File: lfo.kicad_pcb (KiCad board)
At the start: 2 copper layers, 103.7 x 33.7 mm, 36 parts, among them J1 PJ398SM-12 (Tri), J2 PJ398SM-12 (square), J3 PJ398SM-12 (weird), J4 Conn_02x05_Odd_Even, Q1 BC547, SW1 SW_SPDT, U1 TL084

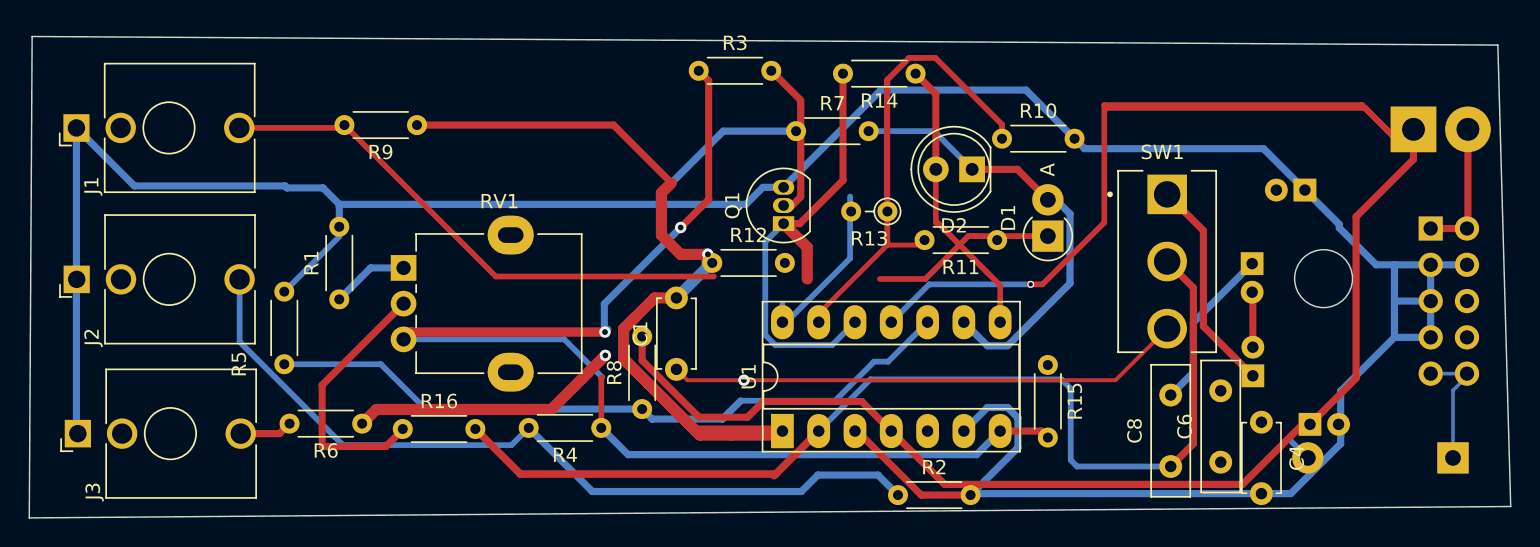
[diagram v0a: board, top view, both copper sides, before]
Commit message: successcive editing
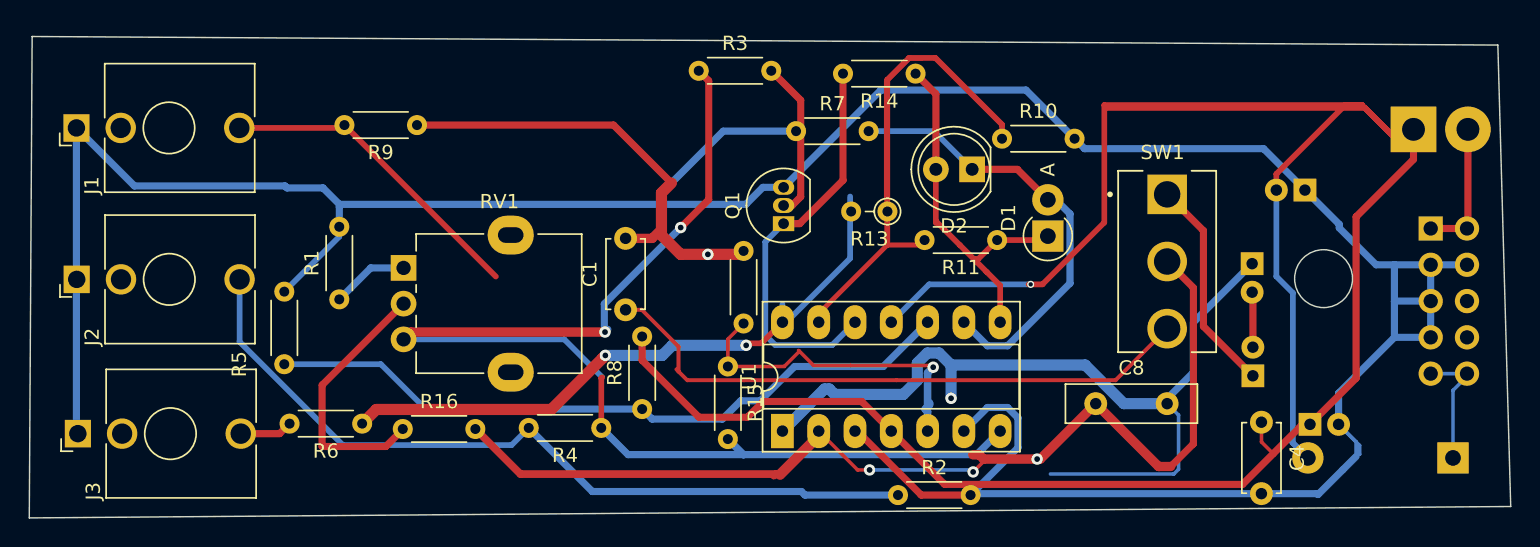
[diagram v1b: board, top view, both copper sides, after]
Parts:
- removed C6: 100nFC, Capacitor_THT:C_Disc_D9.0mm_W2.5mm_P5.00mm
- moved R15 22.4 mm to (105.8, 34.2)
- moved C8 6.85 mm to (131.6, 36.8), turned to 0 degrees
- moved C1 5.48 mm to (98.6, 30.2)
- moved R12 2.35 mm to (106.9, 26.1), turned to -90 degrees
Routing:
- net Vee: track 70.1 -> 98.9 mm
- net Net-(U1B-+): track 0.00 -> 24.3 mm, vias 0 -> 1
- net Net-(C1-Pad2): track 87.4 -> 103.0 mm, vias 1 -> 2
- net Net-(J1-PadT): track 37.7 -> 22.4 mm
- net Net-(R13-Pad2): track 31.2 -> 44.6 mm, vias 1 -> 2
- net Net-(D1-K): track 33.5 -> 25.8 mm
- net Net-(SW1-B): track 96.6 -> 103.7 mm, vias 0 -> 3
- net GND: track 215.5 -> 222.1 mm
- net Net-(SW1-C): track 36.2 -> 42.7 mm, vias 1 -> 0
- net Net-(Q1-C): track 33.0 -> 28.5 mm
- net Vcc: track 78.3 -> 80.9 mm
- net Net-(R15-Pad2): track 111.5 -> 109.5 mm
- net Net-(J2-PadT): track 56.9 -> 55.9 mm

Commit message: fix drc errors
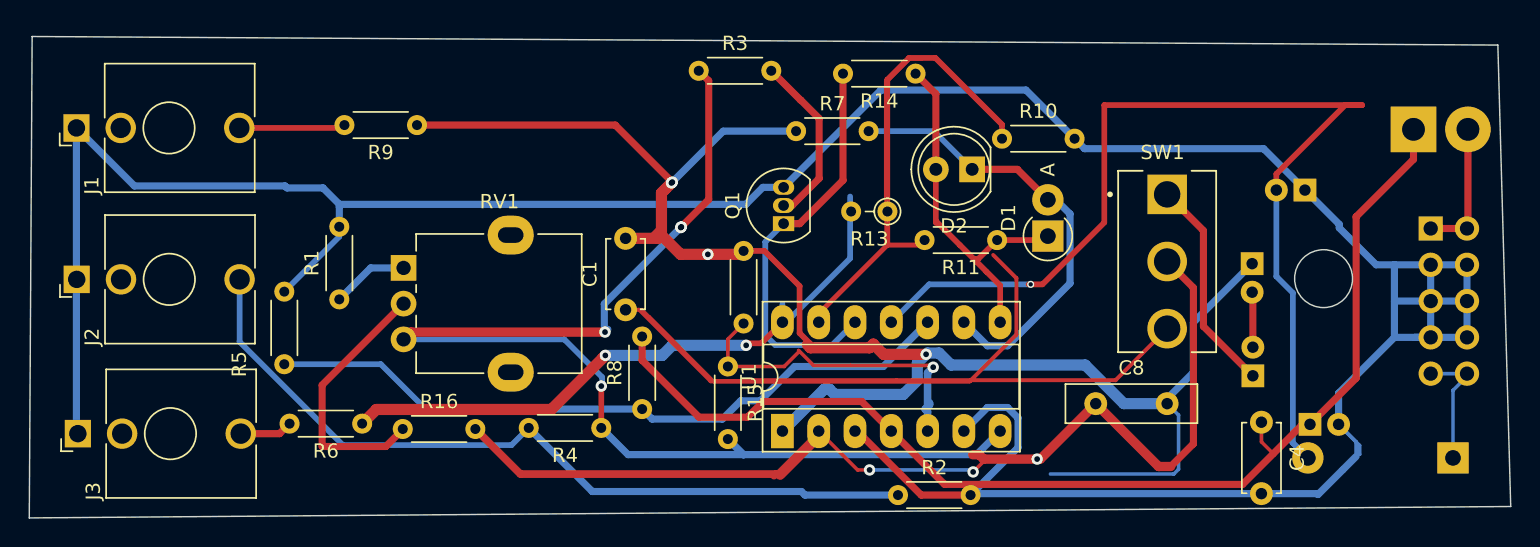
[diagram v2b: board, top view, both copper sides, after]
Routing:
- net Net-(SW1-C): track 42.7 -> 96.1 mm
- net Vee: track 98.9 -> 74.6 mm
- net Net-(C1-Pad2): track 103.0 -> 121.9 mm, vias 2 -> 4
- net Net-(J1-PadT): track 22.4 -> 7.44 mm
- net GND: track 222.1 -> 233.4 mm
- net Net-(Q1-B): track 11.1 -> 12.2 mm
- net Net-(R15-Pad2): vias 2 -> 4
